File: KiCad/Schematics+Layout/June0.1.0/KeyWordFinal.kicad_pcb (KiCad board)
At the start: 2 copper layers, 55 parts, among them J1 USB4105-GF-A, J2 Conn_01x02_Pin, J3 Conn_01x05_Pin, J4 MSD-10-C, U1 NRF52805-CAAA-R, U2 NPM1100-CAAA-R7, U3 TXB0104RUTR, U4 TPS62743YFPR, U5 MCP6142T-E/MS, Y1 32.768k, Y3 32M

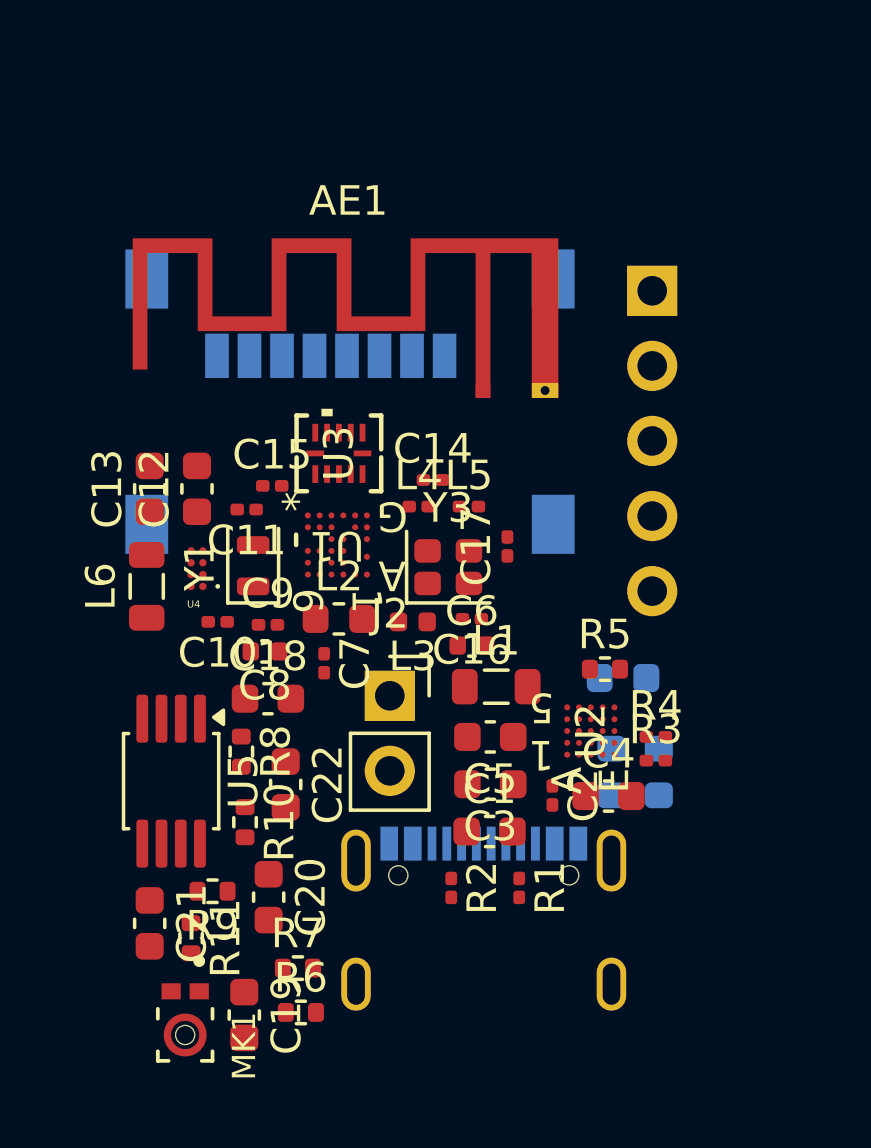
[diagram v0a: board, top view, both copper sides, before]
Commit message: Updated layout, updated schematic to ease layout.
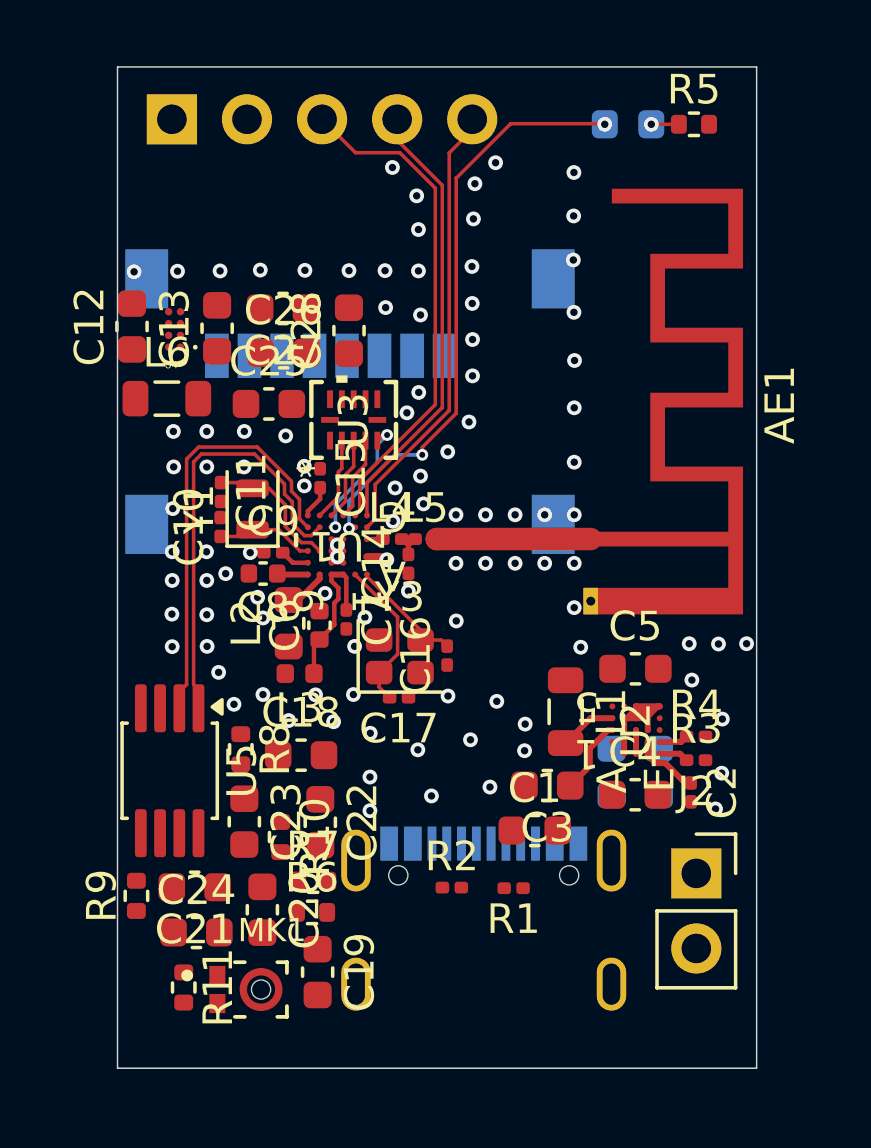
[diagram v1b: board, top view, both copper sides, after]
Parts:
- added C23: 0.1u, Capacitor_SMD:C_0603_1608Metric, F.Cu at (133.2, 73.7)
- added C24: 0.1u, Capacitor_SMD:C_0603_1608Metric, F.Cu at (131.6, 77.4)
- added C25: 0.1u, Capacitor_SMD:C_0603_1608Metric, F.Cu at (134.0, 59.5)
- added C26: 0.1u, Capacitor_SMD:C_0603_1608Metric, F.Cu at (134.5, 57.8)
- added C27: 1.0u, Capacitor_SMD:C_0603_1608Metric, F.Cu at (134.5, 56.3)
- added C28: 0.1u, Capacitor_SMD:C_0603_1608Metric, F.Cu at (136.7, 57.0)
- C19: value C -> 10n
- R6, R7: value R -> 100k
- moved D3 18.7 mm to (146.2, 50.1), turned to 180 degrees
- moved R5 18.7 mm to (148.4, 50.1)
- moved J3 17.3 mm to (130.8, 49.9), turned to -90 degrees
- moved J2 12.0 mm to (148.5, 75.4)
- moved U4 8.13 mm to (130.8, 57.0)
- moved L6 6.39 mm to (130.6, 59.3), turned to 0 degrees
- moved C17 6.29 mm to (138.4, 69.5), turned to 180 degrees
- moved AE1 6.21 mm to (144.9, 64.1), turned to -90 degrees
- moved C12 5.92 mm to (129.4, 56.9)
- moved C13 5.89 mm to (132.3, 57.0)
- moved C5 5.42 mm to (146.4, 68.5), turned to 0 degrees
- moved C6 5.20 mm to (135.7, 67.0), turned to 90 degrees
- moved C2 4.69 mm to (148.3, 72.7)
- moved L3 4.21 mm to (135.1, 68.6)
- moved Y3 3.43 mm to (138.5, 68.1)
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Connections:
- U1 pad F2: Net-(U1-P0.20) -> Net-(D3-A)
- U1 pad F4: Net-(D3-A) -> Net-(U1-P0.14)
- U1 pad F5: VCOM -> /ADC+
- U1 pad F6: /ADC+ -> VCOM
- U3 pad 11: Net-(J4-CLK) -> +3V0
- U3 pad 12: Net-(J4-CMD) -> +1V8
- U3 pad 2: Net-(U1-P0.20) -> Net-(U1-P0.12)
- U3 pad 3: Net-(U1-P0.18) -> Net-(U1-P0.16)
- U3 pad 4: Net-(U1-P0.16) -> Net-(U1-P0.18)
- U3 pad 5: Net-(U1-P0.12) -> Net-(U1-P0.14)
- U3 pad 6: unconnected-(U3-NC-Pad6) -> GND
- U3 pad 7: GND -> Net-(J4-DAT3/CD)
- U3 pad 8: +1V8 -> Net-(J4-CMD)
- U3 pad 9: unconnected-(U3-NC-Pad9) -> Net-(J4-CLK)
- Y3 pad 1: Net-(U1-XC1) -> Net-(U1-XC2)
- Y3 pad 3: Net-(U1-XC2) -> Net-(U1-XC1)
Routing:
- net Net-(D3-A): track 0.00 -> 19.9 mm, vias 0 -> 3
- net Net-(J3-Pin_3): track 0.00 -> 17.0 mm
- net Net-(J3-Pin_5): track 0.00 -> 15.3 mm
- net Net-(J3-Pin_4): track 0.00 -> 15.1 mm
- net /ADC+: track 0.00 -> 14.7 mm
- net VCOM: track 0.00 -> 14.6 mm
- net GND: track 0.00 -> 8.12 mm, vias 0 -> 102
- net Net-(U1-DEC2): track 0.00 -> 5.43 mm
- net /RF: track 0.00 -> 5.21 mm
- net Net-(U1-XC2): track 0.00 -> 5.16 mm
- net Net-(U1-P0.01/XL2): track 0.00 -> 4.74 mm
- net Net-(U1-P0.14): track 0.00 -> 4.39 mm, vias 0 -> 2
- net Net-(U1-XC1): track 0.00 -> 3.96 mm
- net Net-(U1-P0.00/XL1): track 0.00 -> 3.35 mm
- net Net-(U1-P0.12): track 0.00 -> 2.84 mm
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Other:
- board outline added: 21.6 x 33.9 mm
- rule pad_to_mask_clearance: 0 -> 0.0762
